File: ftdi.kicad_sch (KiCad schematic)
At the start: 22 parts, among them U1 FT2232H-56Q, U11 93LC56CT-IMC, Y4 ABM8G-12M-18-D2Y-T

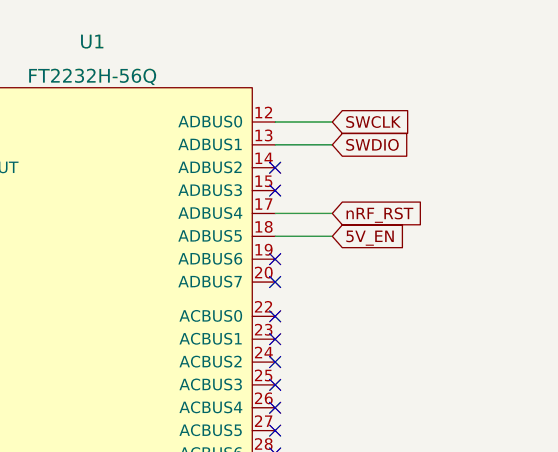
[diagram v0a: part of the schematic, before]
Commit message: Fixed SWD
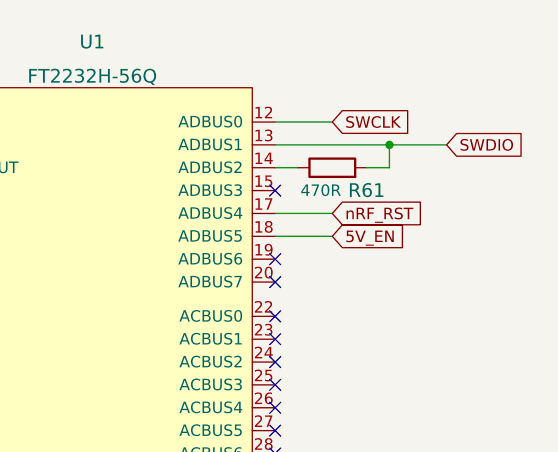
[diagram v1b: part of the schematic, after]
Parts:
- added R61: R_470R_0402, antmicro-footprints:0402-res, symbol antmicroResistors0402:R_470R_0402
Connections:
- net SWDIO: now also R61.2
- net at U1.14 (ADBUS2): now also R61.1
- no-connect marks 28 -> 27
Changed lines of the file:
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@@
   (junction (at 45.72 31.75) (diameter 0) (color 0 0 0 0)
+  )
+  (junction (at 176.53 44.45) (diameter 0) (color 0 0 0 0)
   )
   (junction (at 38.1 41.91) (diameter 0) (color 0 0 0 0)
@@
   (no_connect (at 163.83 97.79))
   (no_connect (at 163.83 124.46))
-  (no_connect (at 163.83 46.99))
   (no_connect (at 163.83 49.53))
   (no_connect (at 163.83 57.15))
@@
     (stroke (width 0) (type default) (color 0 0 0 0))
   )
+  (wire (pts (xy 176.53 44.45) (xy 182.88 44.45))
+    (stroke (width 0) (type default) (color 0 0 0 0))
+  )
   (wire (pts (xy 85.09 93.98) (xy 92.71 93.98))
     (stroke (width 0) (type default) (color 0 0 0 0))
@@
     (stroke (width 0) (type default) (color 0 0 0 0))
   )
-  (wire (pts (xy 163.83 44.45) (xy 170.18 44.45))
+  (wire (pts (xy 163.83 44.45) (xy 176.53 44.45))
     (stroke (width 0) (type default) (color 0 0 0 0))
   )
@@
     (stroke (width 0) (type default) (color 0 0 0 0))
   )
+  (wire (pts (xy 176.53 46.99) (xy 176.53 44.45))
+    (stroke (width 0) (type default) (color 0 0 0 0))
+  )
   (wire (pts (xy 73.66 31.75) (xy 81.28 31.75))
     (stroke (width 0) (type default) (color 0 0 0 0))
@@
     (stroke (width 0) (type default) (color 0 0 0 0))
   )
+  (wire (pts (xy 163.83 46.99) (xy 166.37 46.99))
+    (stroke (width 0) (type default) (color 0 0 0 0))
+  )
   (wire (pts (xy 81.28 41.91) (xy 88.9 41.91))
     (stroke (width 0) (type default) (color 0 0 0 0))
@@
   )
   (wire (pts (xy 83.82 93.98) (xy 85.09 93.98))
+    (stroke (width 0) (type default) (color 0 0 0 0))
+  )
+  (wire (pts (xy 173.99 46.99) (xy 176.53 46.99))
     (stroke (width 0) (type default) (color 0 0 0 0))
   )
@@
     )
   )
-  (global_label "SWDIO" (shape input) (at 170.18 44.45 0) (fields_autoplaced)
+  (global_label "SWDIO" (shape input) (at 182.88 44.45 0) (fields_autoplaced)
     (effects (font (size 1.27 1.27)) (justify left))
-    (property "Intersheet References" "${INTERSHEET_REFS}" (id 0) (at 178.3704 44.3706 0)
+    (property "Intersheet References" "${INTERSHEET_REFS}" (id 0) (at 191.0704 44.3706 0)
       (effects (font (size 1.27 1.27)) (justify left) hide)
     )
@@
     (pin "1")
   )
+  (symbol (lib_id "antmicroResistors0402:R_470R_0402") (at 170.18 46.99 0) (unit 1)
+    (in_bom yes) (on_board yes)
+    (property "Reference" "R61" (id 0) (at 173.99 49.53 0)
+      (effects (font (size 1.524 1.524)))
+    )
+    (property "Value" "R_470R_0402" (id 1) (at 170.18 50.8 0)
+      (effects (font (size 1.524 1.524)) hide)
+    )
+    (property "Footprint" "antmicro-footprints:0402-res" (id 2) (at 175.26 41.91 0)
+      (effects (font (size 1.524 1.524)) (justify left) hide)
+    )
+    (property "Datasheet" "" (id 3) (at 170.18 46.99 0)
+      (effects (font (size 1.27 1.27)) hide)
+    )
+    (property "Manufacturer" "VISHAY" (id 4) (at 175.26 36.83 0)
+      (effects (font (size 1.524 1.524)) (justify left) hide)
+    )
+    (property "MPN" "CRCW0402470RFKED" (id 5) (at 175.26 39.37 0)
+      (effects (font (size 1.524 1.524)) (justify left) hide)
+    )
+    (property "Val" "470R" (id 6) (at 168.91 49.53 0))
+    (pin "1")
+    (pin "2")
+  )
   (symbol (lib_id "antmicroMemory:93LC56CT-IMC") (at 69.85 111.76 0) (unit 1)
